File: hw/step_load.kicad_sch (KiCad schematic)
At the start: 59 parts, among them J1 DC_IN, J2 USB_C_Receptacle_USB2.0_16P, J3 OUTPUT, J4 OLED, J5 UART, J6 BOOT, J7 DC_IN, SW1 RST, SW2 RST, SW3 RST, SW4 RST, U1 AZ1117-3.3, U2 TCA9535PWR, U3 LM35DZ, U4 LM35DZ, U5 ESP32-C3-WROOM-02

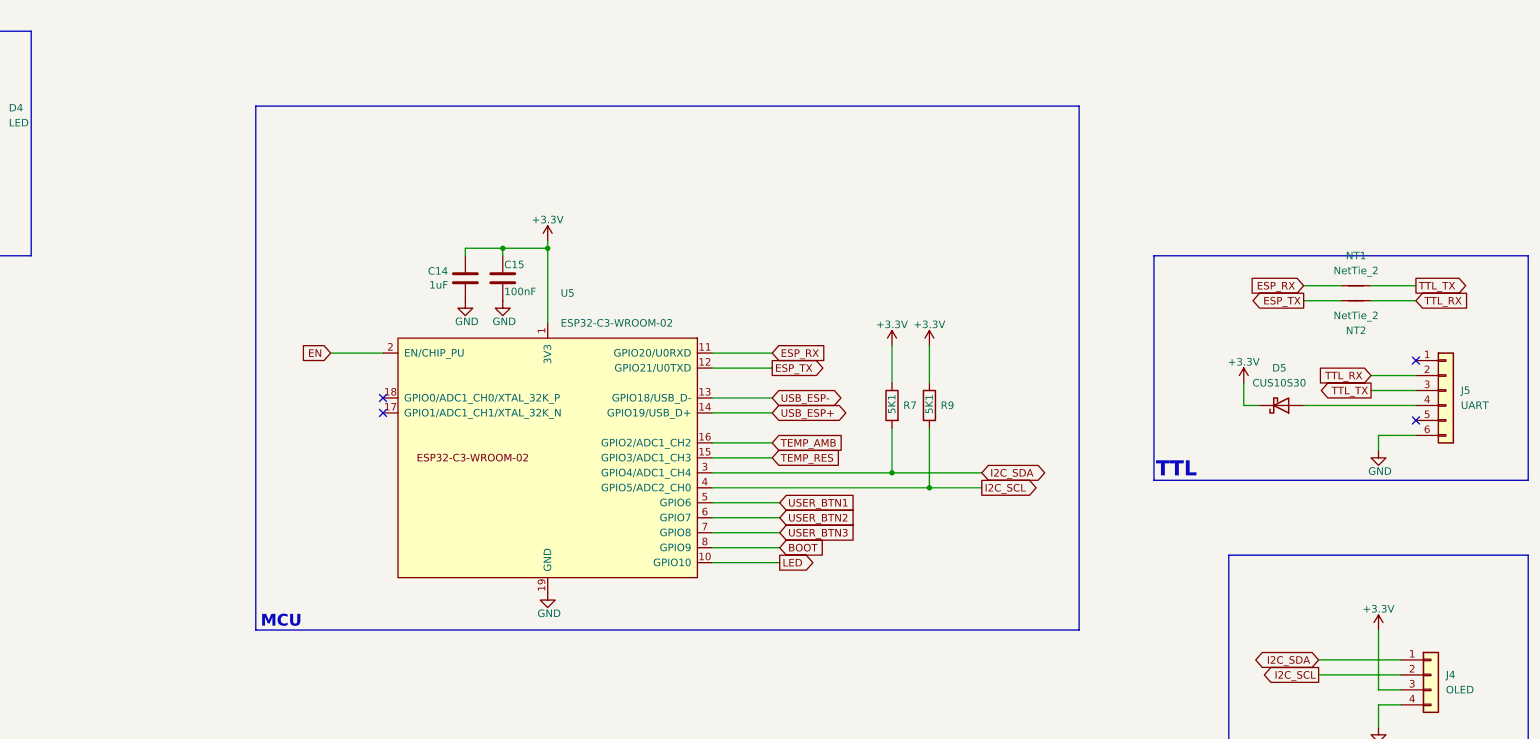
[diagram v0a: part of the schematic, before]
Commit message: sch & pcb update
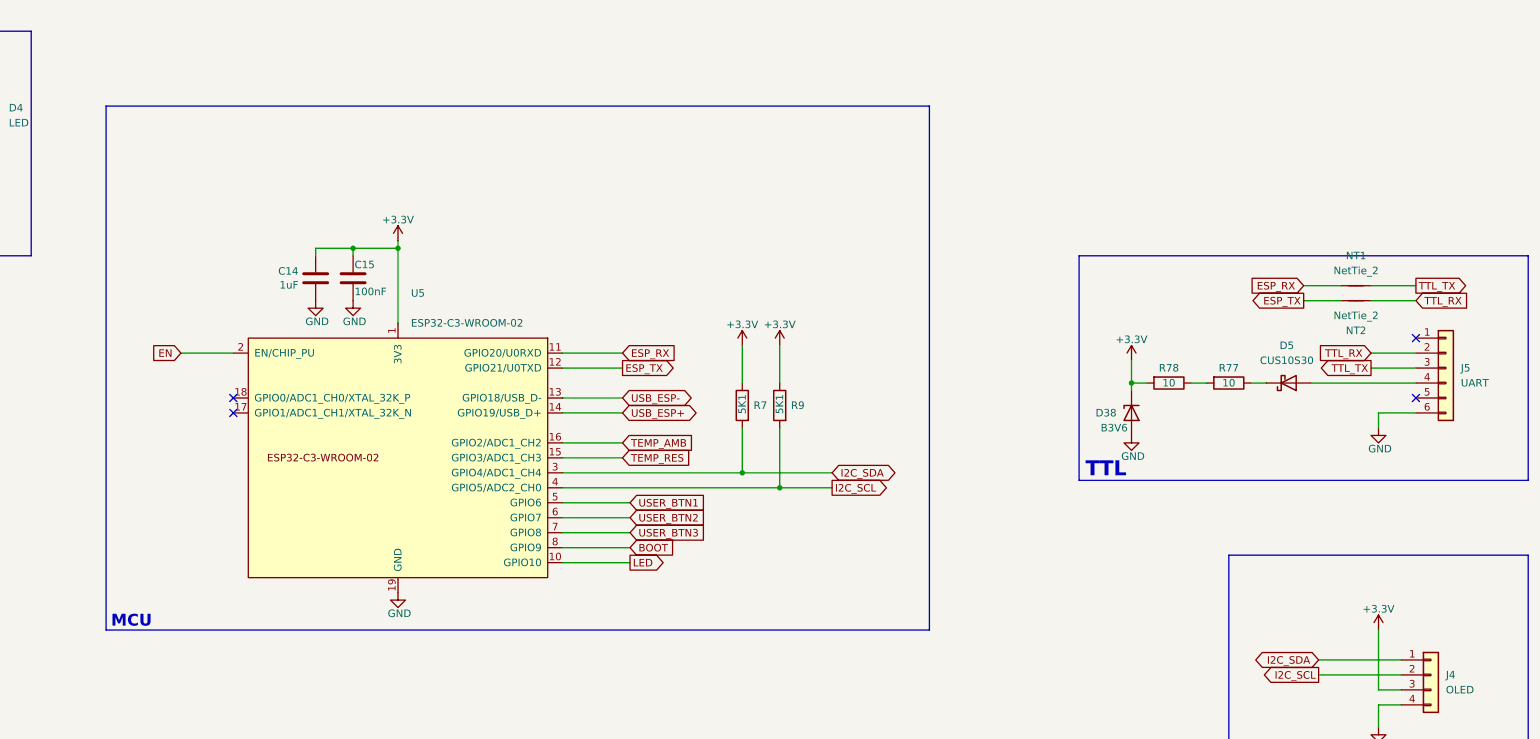
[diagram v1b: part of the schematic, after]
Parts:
- added D38: B3V6, Diode_SMD:D_SOD-523, symbol Device:D_Zener
- added R77, R78: 10, Resistor_SMD:R_0603_1608Metric, symbol Device:R
- R2, R3, R7, R9: jlc_part (none) -> C23186; mfr_part (none) -> 0603WAF5101T5E
- R4, R5: jlc_part C118155 -> C21190; mfr_part ERJ3EKF1001V -> 0603WAF1001T5E
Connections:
- net +3.3V: now also D38.1 (K), R78.2; no longer D5.1 (K)
- net GND: now also D38.2 (A)
- new net: D5.1 (K), R77.1
- new net: R77.2, R78.1
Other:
- moved on the sheet: C14, C15, D5, J5, R7, R9, U5
